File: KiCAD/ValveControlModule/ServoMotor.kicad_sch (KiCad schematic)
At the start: 5 parts, among them J1 DF51A-4P-2DS, U2 LT1785xS8

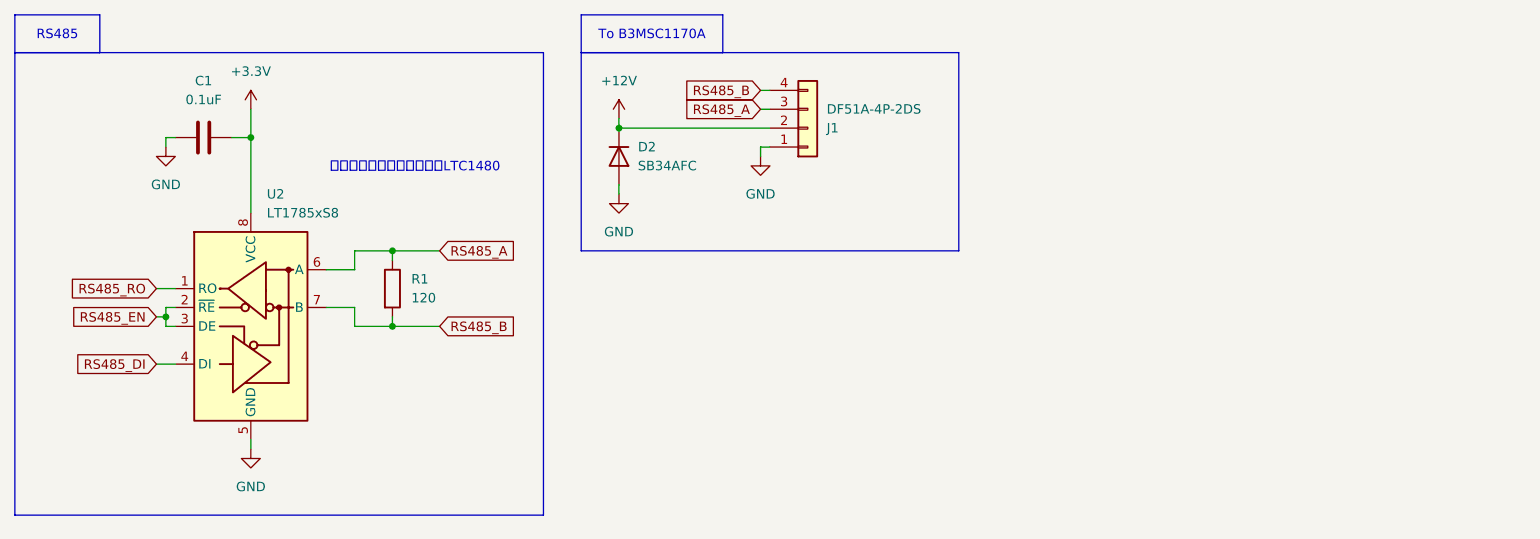
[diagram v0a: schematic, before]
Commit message: Build-2完成．発注．
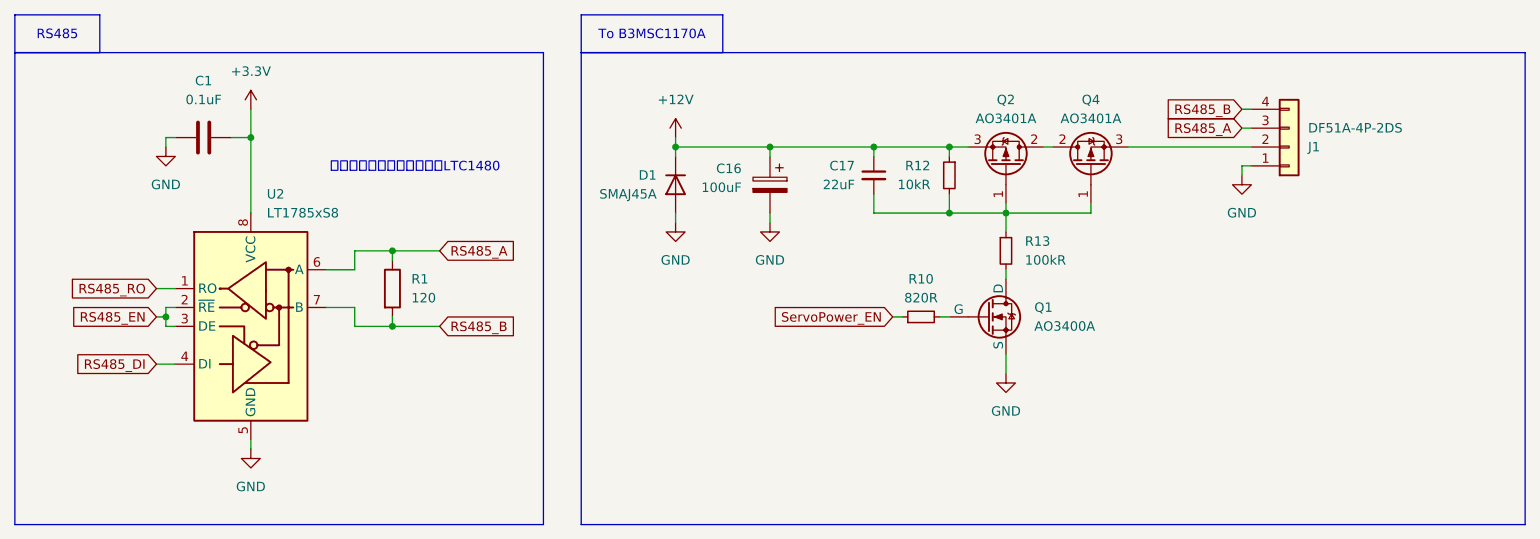
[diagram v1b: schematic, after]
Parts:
- removed D2: SB34AFC, Diode_SMD:D_SMA_Handsoldering, symbol Device:D
- added C16: 100uF, Capacitor_THT:CP_Radial_D8.0mm_P3.50mm, symbol Device:C_Polarized
- added C17: 22uF, Capacitor_SMD:C_0805_2012Metric_Pad1.18x1.45mm_HandSolder, symbol Device:C_Small
- added D1: SMAJ45A, Diode_SMD:D_SMA, symbol Device:D
- added Q1: AO3400A, Package_TO_SOT_SMD:SOT-23_Handsoldering, symbol Simulation_SPICE:NMOS
- added Q2, Q4: AO3401A, Package_TO_SOT_SMD:SOT-23_Handsoldering, symbol Transistor_FET:QM6015D
- added R10: 820R, Resistor_SMD:R_0603_1608Metric_Pad0.98x0.95mm_HandSolder, symbol Device:R_Small
- added R12: 10kR, Resistor_SMD:R_0603_1608Metric_Pad0.98x0.95mm_HandSolder, symbol Device:R_Small
- added R13: 100kR, Resistor_SMD:R_0603_1608Metric_Pad0.98x0.95mm_HandSolder, symbol Device:R_Small
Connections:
- net +12V: now also C16.1, C17.1, D1.1 (K), Q2.3 (S), R12.1; no longer J1.2 (Pin_2)
- net GND: now also C16.2, D1.2 (A), Q1.3 (S)
- new net: C17.2, Q2.1 (G), Q4.1 (G), R12.2, R13.1
- new net: Q2.2 (D), Q4.2 (D)
- new net: Q1.1 (D), R13.2
- new net: Q1.2 (G), R10.2
- new net: J1.2 (Pin_2), Q4.3 (S)
- new net ServoPower_EN: R10.1
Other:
- moved on the sheet: J1
